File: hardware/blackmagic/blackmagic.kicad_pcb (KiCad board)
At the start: 4 copper layers, 49 x 40 mm, 59 parts, among them Q1 2N7002, Q2 AO3401A, SW1 TS-1187A-B-A-B, SW2 TS-1187A-B-A-B, SW3 TS-1187A-B-A-B, U1 STM32F411CEUx, U2 USBLC6-2P6, U3 AP2112K-3.3TRG1, U4 TXS0108ERGYR, X1 32.768kHz crystal, X2 25Mhz crystal

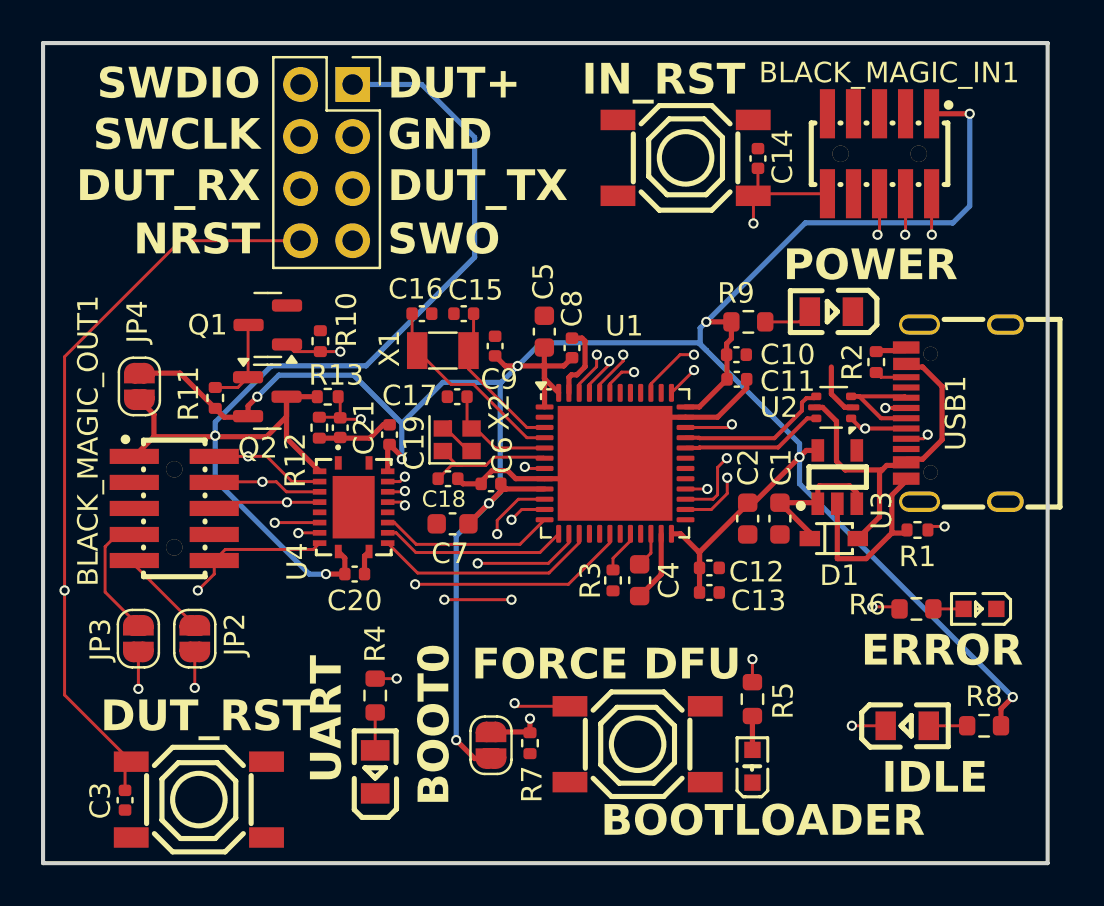
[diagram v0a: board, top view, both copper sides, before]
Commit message: Run cleanup pass
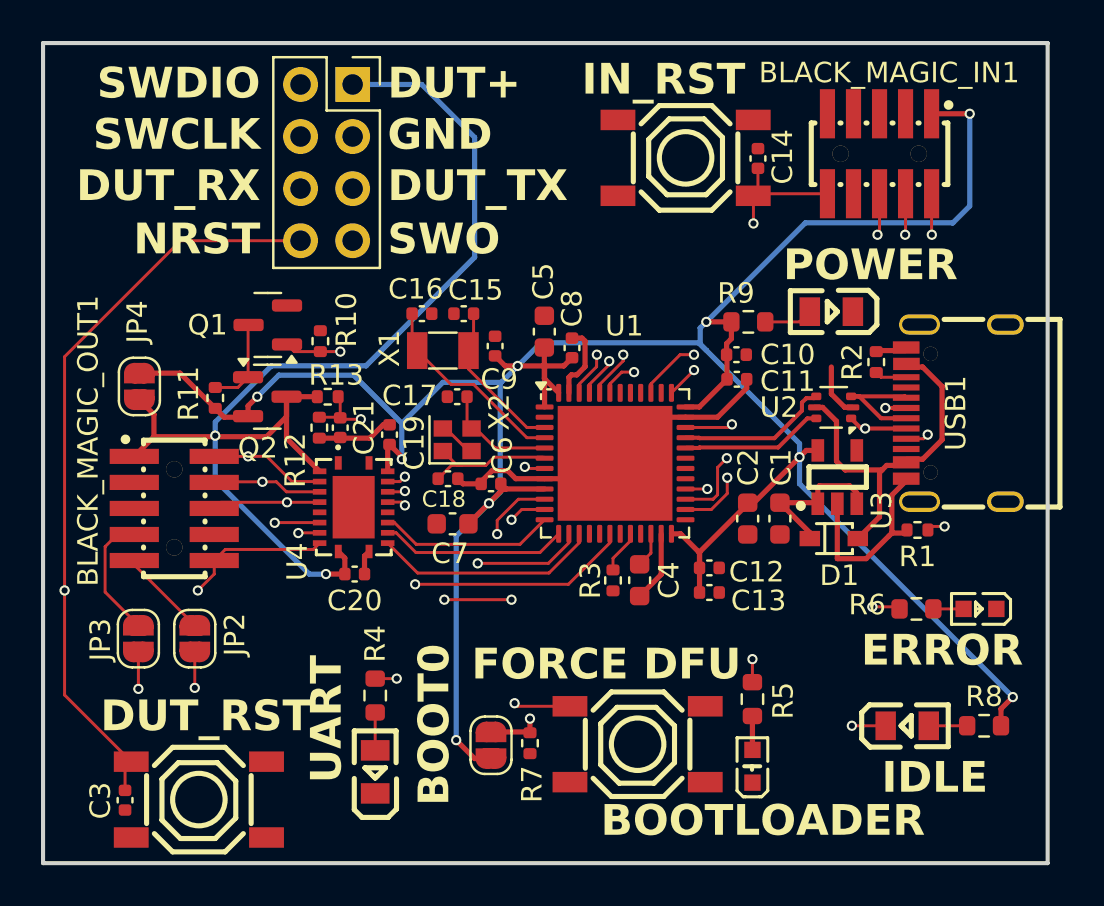
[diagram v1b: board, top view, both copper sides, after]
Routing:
- net GND: track 44.9 -> 39.7 mm
- net Net-(JP2-A): track 6.18 -> 5.35 mm
- net +3V3: track 137.4 -> 136.8 mm
- net /OSC_IN: track 5.60 -> 5.09 mm
